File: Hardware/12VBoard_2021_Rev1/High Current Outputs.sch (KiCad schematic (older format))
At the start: 8 parts

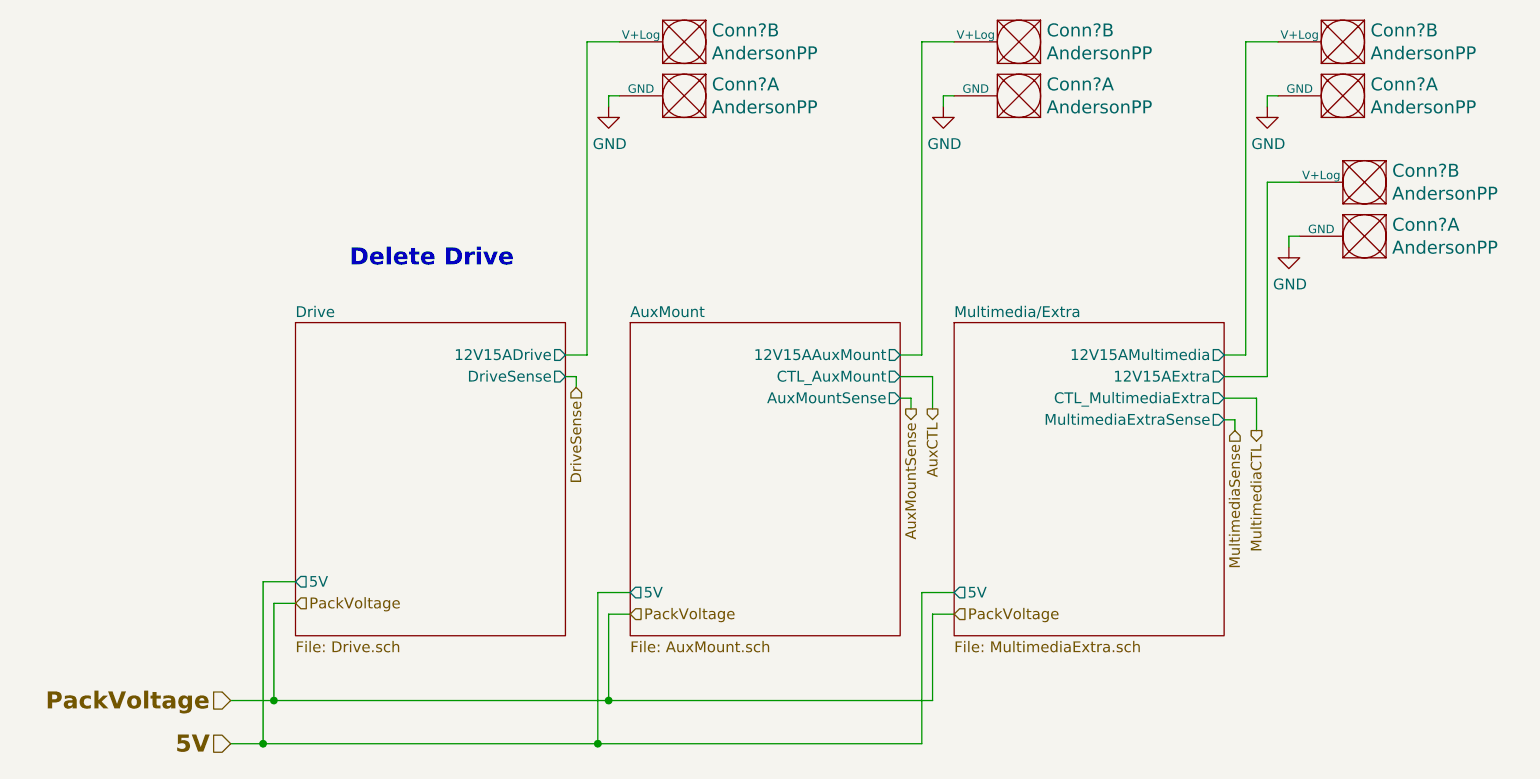
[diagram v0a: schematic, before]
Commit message: reviewed
review
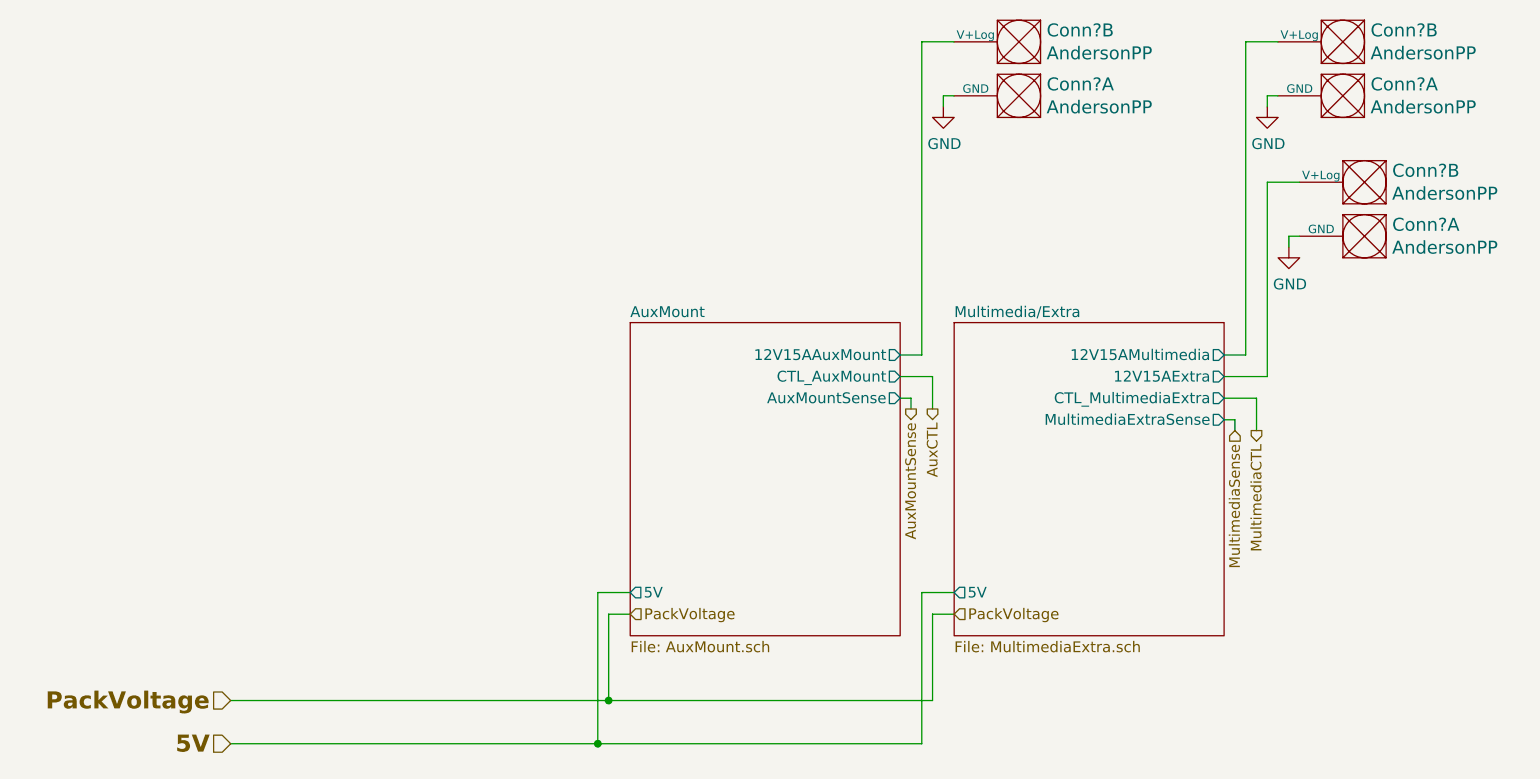
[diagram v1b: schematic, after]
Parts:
- removed Conn? (x2): AndersonPP, symbol MRDT_Connectors:AndersonPP
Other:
- note removed: "Delete Drive"
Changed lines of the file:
@@
 $Descr A4 11693 8268
 encoding utf-8
-Sheet 5 8
+Sheet 5 7
 Title ""
 Date ""
@@
 Text HLabel 1400 4700 0    79   Input ~ 16
 PackVoltage
-Text HLabel 1700 4250 2    50   Input ~ 0
-PackVoltage
 Text HLabel 3250 4300 2    50   Input ~ 0
 PackVoltage
@@
 PackVoltage
 Wire Wire Line
-	1400 4700 1600 4700
-Wire Wire Line
-	1700 4250 1600 4250
-Wire Wire Line
-	1600 4250 1600 4700
-Connection ~ 1600 4700
-Wire Wire Line
 	4650 4700 4650 4300
 Wire Wire Line
 	4650 4300 4750 4300
-Wire Wire Line
-	1600 4700 3150 4700
 Wire Wire Line
 	3250 4300 3150 4300
@@
 Wire Wire Line
 	3150 4700 4650 4700
-$Sheet
-S 1700 2950 1250 1450
-U 5F821EB2
-F0 "Drive" 50
-F1 "Drive.sch" 50
-F2 "12V15ADrive" O R 2950 3100 50
-F3 "DriveSense" O R 2950 3200 50
-F4 "5V" O L 1700 4150 49
-$EndSheet
 $Sheet
 S 4750 2950 1250 1450
@@
 F6 "5V" O L 4750 4200 49
 $EndSheet
-$Comp
-L MRDT_Connectors:AndersonPP Conn?
-U 1 1 5F9BB8B5
-P 3600 1800
-AR Path="/5F74F36B/5F821EB2/5F9BB8B5" Ref="Conn?"  Part="1"
-AR Path="/5F74F36B/5F9BB8B5" Ref="Conn?"  Part="1"
-F 0 "Conn?" H 3572 1847 60  0000 R CNN
-F 1 "AndersonPP" H 3572 1953 60  0000 R CNN
-F 2 "" H 3450 1250 60  0001 C CNN
-F 3 "" H 3450 1250 60  0001 C CNN
-	1    3600 1800
-	-1   0    0    1
-$EndComp
-$Comp
-L MRDT_Connectors:AndersonPP Conn?
-U 2 1 5F9BB8BB
-P 3600 1550
-AR Path="/5F74F36B/5F821EB2/5F9BB8BB" Ref="Conn?"  Part="2"
-AR Path="/5F74F36B/5F9BB8BB" Ref="Conn?"  Part="2"
-F 0 "Conn?" H 3572 1597 60  0000 R CNN
-F 1 "AndersonPP" H 3572 1703 60  0000 R CNN
-F 2 "" H 3450 1000 60  0001 C CNN
-F 3 "" H 3450 1000 60  0001 C CNN
-	2    3600 1550
-	-1   0    0    1
-$EndComp
-$Comp
-L power:GND #PWR?
-U 1 1 5F9BB8C1
-P 3150 1950
-AR Path="/5F74F36B/5F821EB2/5F9BB8C1" Ref="#PWR?"  Part="1"
-AR Path="/5F74F36B/5F9BB8C1" Ref="#PWR?"  Part="1"
-F 0 "#PWR?" H 3150 1700 50  0001 C CNN
-F 1 "GND" H 3155 1777 50  0000 C CNN
-F 2 "" H 3150 1950 50  0001 C CNN
-F 3 "" H 3150 1950 50  0001 C CNN
-	1    3150 1950
-	1    0    0    -1
-$EndComp
-Wire Wire Line
-	3200 1900 3150 1900
-Wire Wire Line
-	3150 1900 3150 1950
-Wire Wire Line
-	2950 3100 3050 3100
-Wire Wire Line
-	3050 3100 3050 1650
-Wire Wire Line
-	3050 1650 3200 1650
 $Comp
 L MRDT_Connectors:AndersonPP Conn?
@@
 $EndSheet
 Wire Wire Line
-	1400 4900 1550 4900
-Wire Wire Line
 	4600 4900 4600 4200
 Wire Wire Line
@@
 Wire Wire Line
 	3100 4900 4600 4900
-Wire Wire Line
-	1700 4150 1550 4150
-Wire Wire Line
-	1550 4150 1550 4900
-Connection ~ 1550 4900
-Wire Wire Line
-	1550 4900 3100 4900
-Text Notes 1950 2700 0    79   ~ 16
-Delete Drive
 Text HLabel 4650 3350 3    49   Output ~ 0
 AuxCTL
@@
 Wire Wire Line
 	6150 3300 6150 3450
-Text HLabel 3000 3250 3    49   Input ~ 0
-DriveSense
-Wire Wire Line
-	3000 3250 3000 3200
-Wire Wire Line
-	3000 3200 2950 3200
+Wire Wire Line
+	1400 4700 3150 4700
+Wire Wire Line
+	1400 4900 3100 4900
 $EndSCHEMATC
